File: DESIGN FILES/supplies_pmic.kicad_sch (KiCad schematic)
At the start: 29 parts

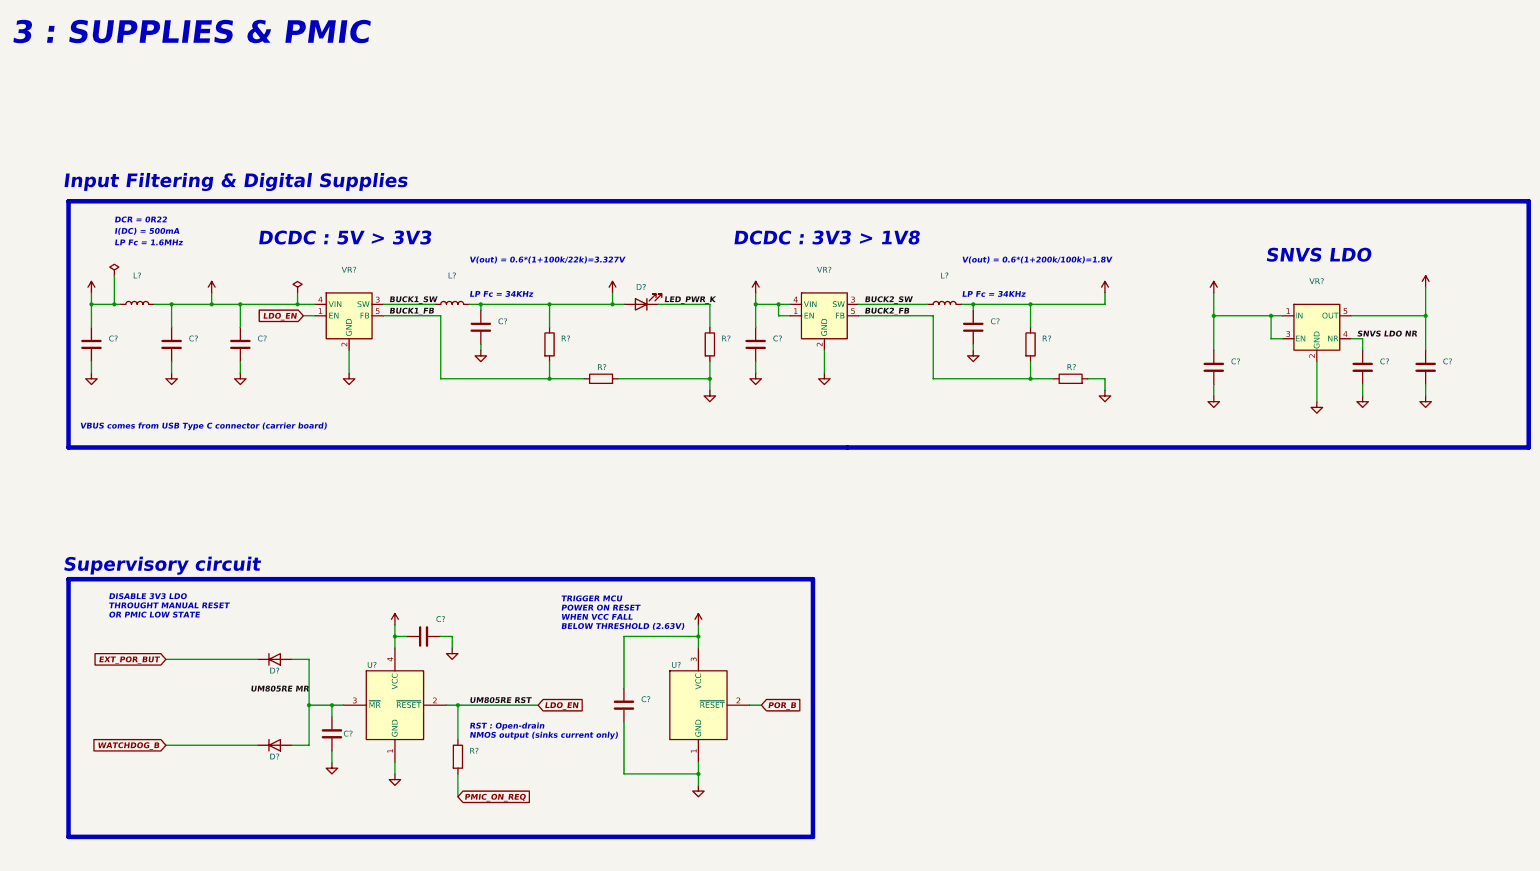
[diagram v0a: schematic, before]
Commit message: schematic changes
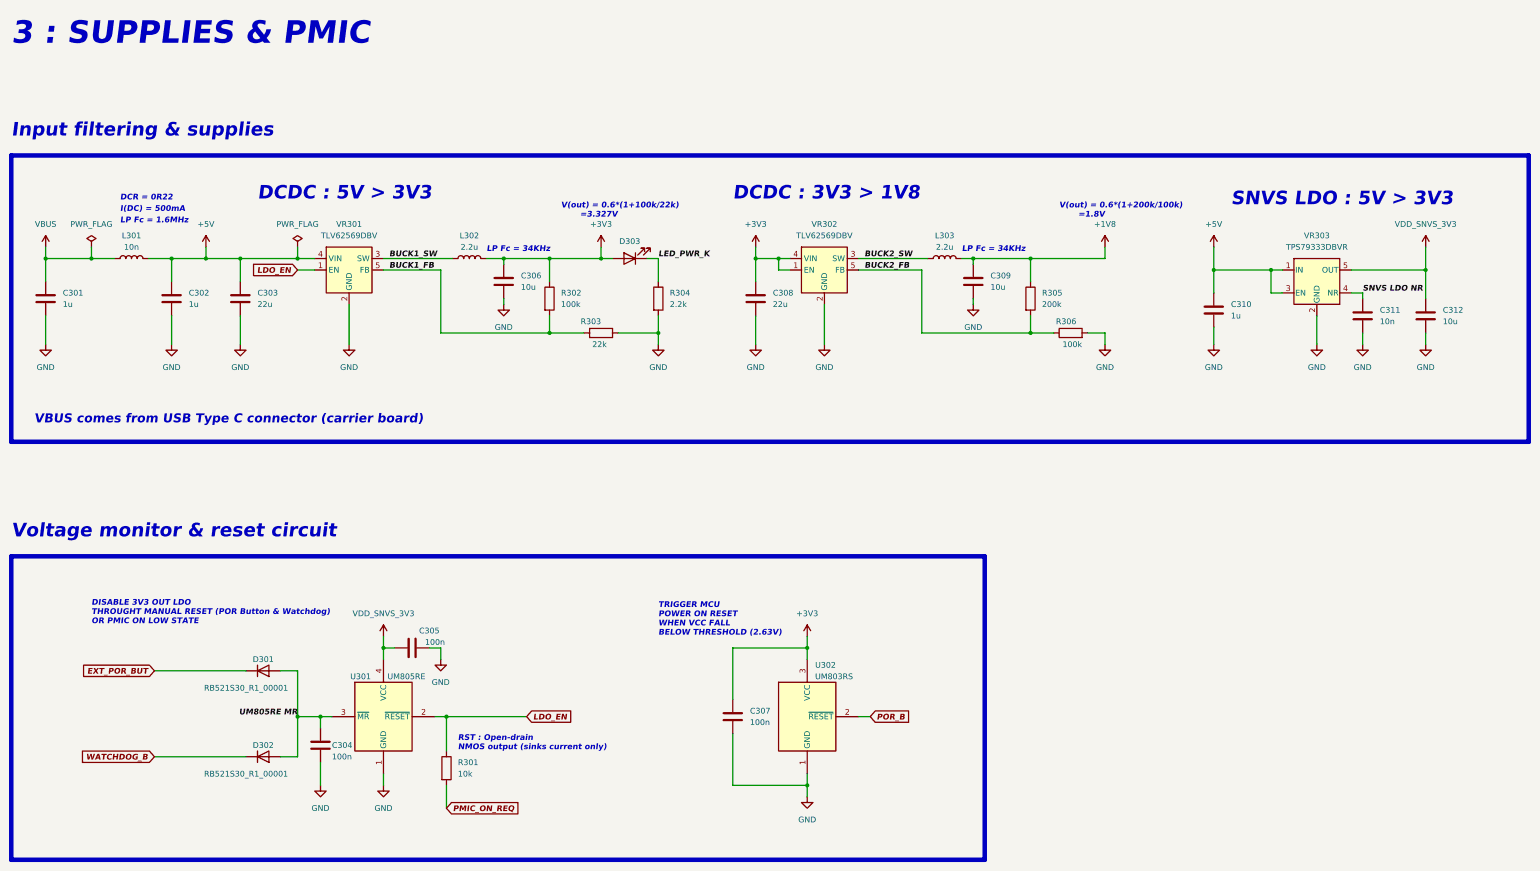
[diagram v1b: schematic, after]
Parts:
- removed C?: ~, symbol MIMXRT1064 MCU Module:CL05A105KA5NQNC
- removed U?: ~, symbol MIMXRT1064 MCU Module:UM803RS
- added C301: 1u, symbol MIMXRT1064 MCU Module:CL05A105KA5NQNC
- added U302: UM803RS, symbol MIMXRT1064 MCU Module:UM803RS
- C302, C310: renamed from C?; value ~ -> 1u
- C303, C308: renamed from C?; value ~ -> 22u
- C304, C305, C307: renamed from C?; value ~ -> 100n
- C306, C309, C312: renamed from C?; value ~ -> 10u
- C311: renamed from C?; value ~ -> 10n
- D301, D302: renamed from D?; value ~ -> RB521S30_R1_00001
- L301: renamed from L?; value ~ -> 10n
- L302, L303: renamed from L?; value ~ -> 2.2u
- R301: renamed from R?; value ~ -> 10k
- R302, R306: renamed from R?; value ~ -> 100k
- R303: renamed from R?; value ~ -> 22k
- R304: renamed from R?; value ~ -> 2.2k
- R305: renamed from R?; value ~ -> 200k
- U301: renamed from U?; value ~ -> UM805RE
- VR301, VR302: renamed from VR?; value ~ -> TLV62569DBV
- VR303: renamed from VR?; value ~ -> TPS79333DBVR
- gave numbers to parts that had none: 1
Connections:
- net +3V3: now also U302.3 (VCC)
- net GND: now also C301.2, U302.1 (GND)
- net POR_B: now also U302.2 (~{RESET})
- net VBUS: now also C301.1
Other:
- note added: "DISABLE 3V3 OUT LDO THROUGHT MANUAL RESET (POR Button & Watchdog) OR PMIC ON LOW STATE"
- note added: "Input filtering & supplies"
- note added: "SNVS LDO : 5V > 3V3"
- note added: "V(out) = 0.6*(1+100k/22k) =3.327V"
- note added: "V(out) = 0.6*(1+200k/100k) =1.8V"
- note added: "Voltage monitor & reset circuit"
- note removed: "DISABLE 3V3 LDO THROUGHT MANUAL RESET OR PMIC LOW STATE"
- note removed: "Input Filtering & Digital Supplies"
- note removed: "SNVS LDO"
- note removed: "Supervisory circuit"
- note removed: "V(out) = 0.6*(1+100k/22k)=3.327V"
- note removed: "V(out) = 0.6*(1+200k/100k)=1.8V"
- moved on the sheet: C302, C303, C304, C305, C306, C307, C308, C309, C310, C311, C312, D301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
